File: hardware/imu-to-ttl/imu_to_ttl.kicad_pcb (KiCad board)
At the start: 2 copper layers, 41 x 30 mm, 57 parts, among them J1 BATT IN 2.54 2P, J2 SWD+UART+NRST, J3 J_NECK, J4 J_L, J5 J_R, Q1 AO4407C, U1 STM32G031F8P6, U2 LSM6DSV16XTR, U3 SN74LVC2G241DCUR, U4 HT7533-1

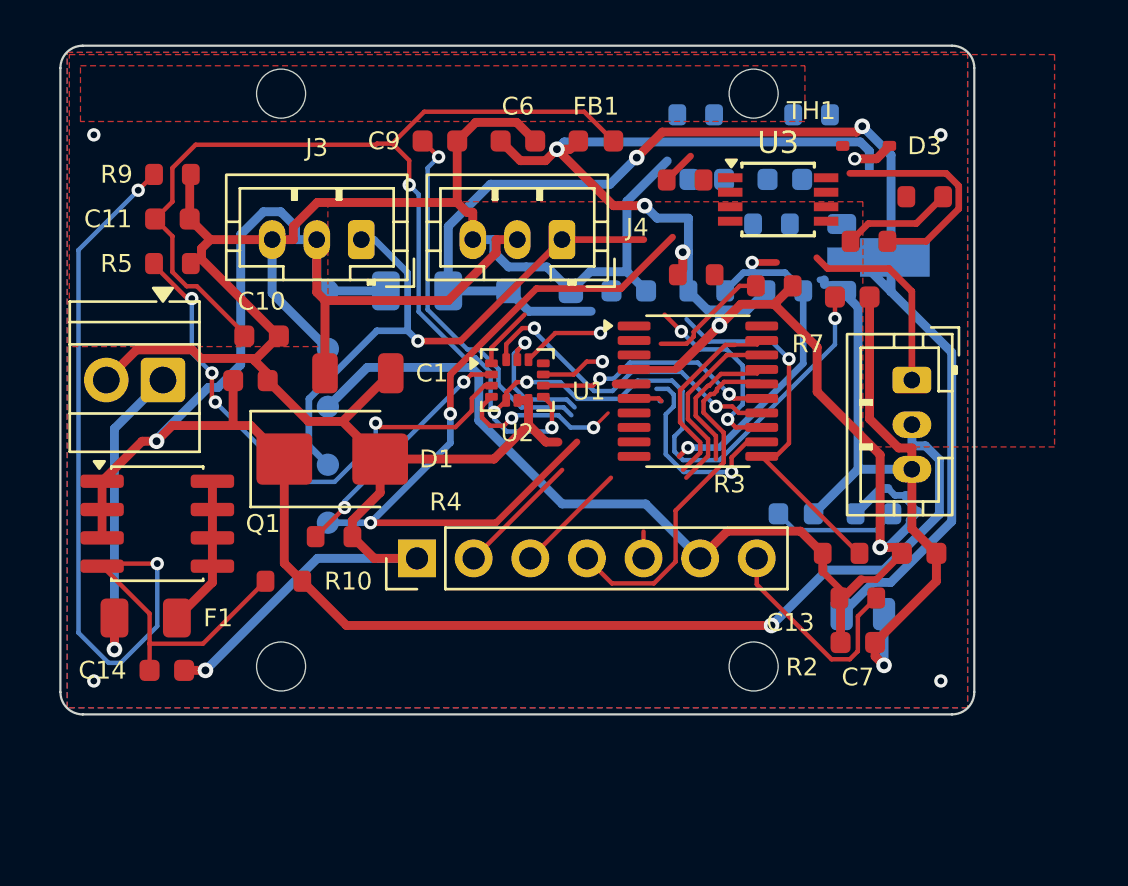
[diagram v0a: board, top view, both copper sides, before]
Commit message: sync: 2026-10-12 日常更新
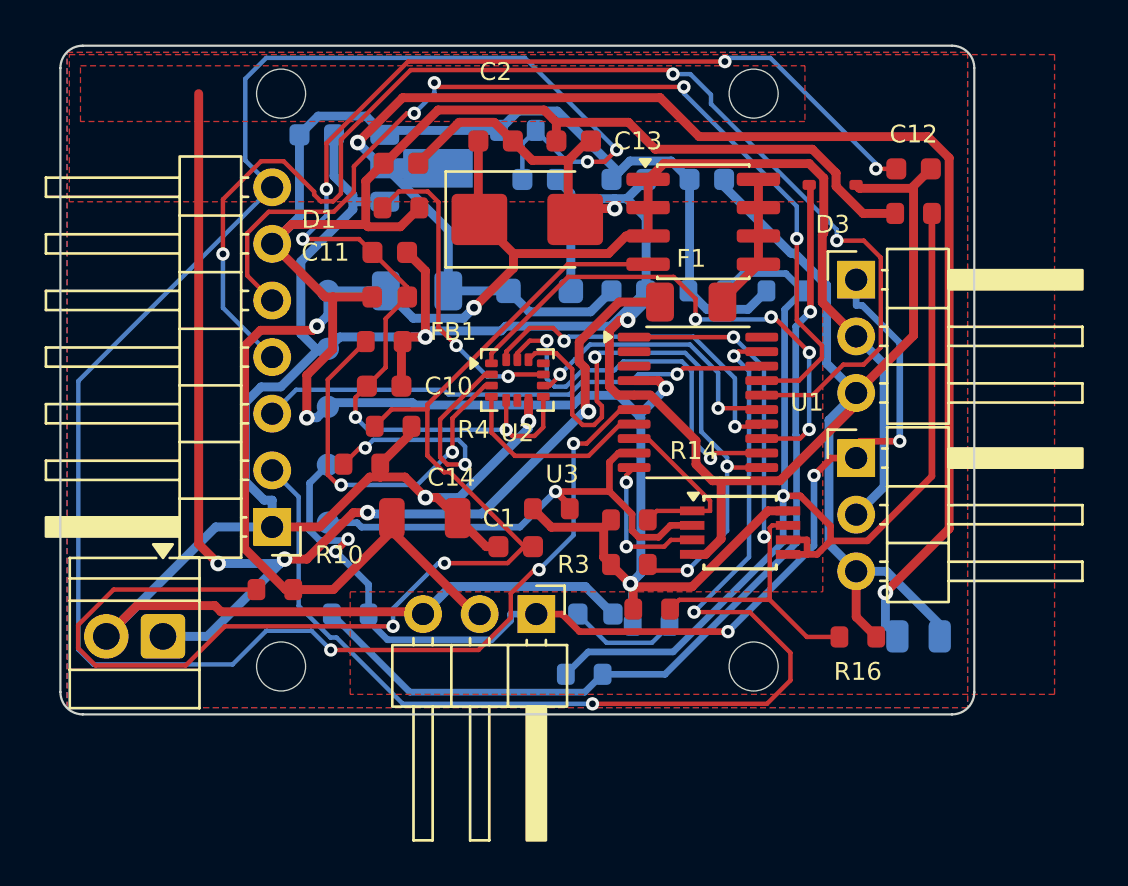
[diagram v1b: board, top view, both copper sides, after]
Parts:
- C6, C9, R13, R2, TH1: moved to B.Cu
- J2: footprint PinHeader_1x07_P2.54mm_Vertical -> PinHeader_1x07_P2.54mm_Horizontal
- J3, J4, J5: footprint JST_PH_B3B-PH-K_1x03_P2.00mm_Vertical -> PinHeader_1x03_P2.54mm_Horizontal
- R14, R15, R16: moved to F.Cu
- U3: footprint Package_SO:TSSOP-8_3x3mm_P0.65mm -> TSSOP-8_3x3mm_P0.65mm
- moved C7 29.7 mm to (15.3, 5.28)
- moved F1 28.3 mm to (28.3, 11.5)
- moved Q1 28.0 mm to (28.8, 7.90)
- moved R2 25.9 mm to (20.5, 3.80)
- moved TH1 24.6 mm to (13.0, 25.5)
- moved R16 24.5 mm to (35.8, 26.5)
- moved C13 24.1 mm to (23.0, 4.28)
- moved R13 23.2 mm to (23.5, 28.2)
- moved C5 21.1 mm to (11.5, 4.00)
- moved U4 20.9 mm to (16.5, 5.50)
- moved R14 19.9 mm to (25.5, 21.3)
- moved J3 18.5 mm to (21.4, 25.5), turned to -90 degrees
- moved R15 18.1 mm to (26.5, 25.3)
- moved R6 17.1 mm to (15.3, 7.28)
- moved C14 16.6 mm to (20.4, 22.5), turned to 180 degrees
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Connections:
- R16 pad 1: GND -> RX_EN
- R16 pad 2: RX_EN -> GND
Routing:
- net NRST: track 28.2 -> 89.1 mm, vias 1 -> 5
- net GND: track 141.6 -> 199.5 mm, vias 7 -> 5
- net VBAT_RAW: track 14.4 -> 55.2 mm, vias 1 -> 4
- net UART1_TX: track 16.4 -> 57.2 mm, vias 0 -> 3
- net UART1_RX: track 7.81 -> 44.7 mm, vias 0 -> 4
- net SWCLK: track 14.5 -> 51.3 mm, vias 0 -> 3
- net BUS_LOGIC: track 21.3 -> 52.5 mm, vias 2 -> 1
- net BUS_CLAMP: track 11.5 -> 41.4 mm, vias 0 -> 1
- net +3V3: track 101.5 -> 129.6 mm, vias 5 -> 3
- net RX_EN: track 0.00 -> 26.8 mm, vias 0 -> 2
- net V3V3_IMU: track 74.7 -> 58.1 mm, vias 5 -> 6
- net VBAT: track 93.7 -> 79.3 mm
- net BUS_DATA: track 35.8 -> 49.1 mm, vias 1 -> 5
- net Q1_GATE: track 44.0 -> 56.6 mm
- net SPI_MISO: track 11.6 -> 23.9 mm, vias 2 -> 4
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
